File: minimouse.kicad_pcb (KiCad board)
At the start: 2 copper layers, 90 x 85 mm, 22 parts, among them J1 Conn_ARM_JTAG_SWD_10, J5 Conn_01x02, M1 N20_encoder, M2 N20_encoder, U1 STM32F030C8Tx, U4 HC-SR04

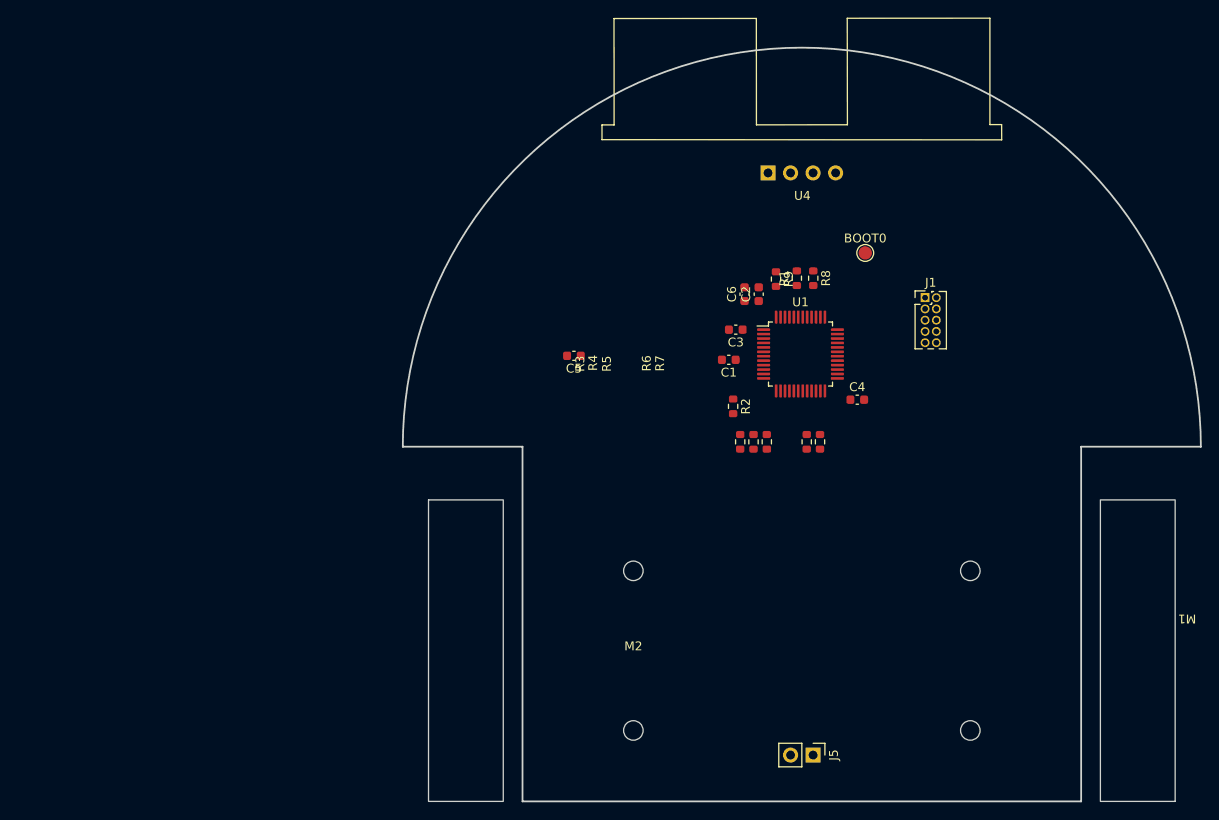
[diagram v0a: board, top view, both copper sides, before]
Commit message: TP2
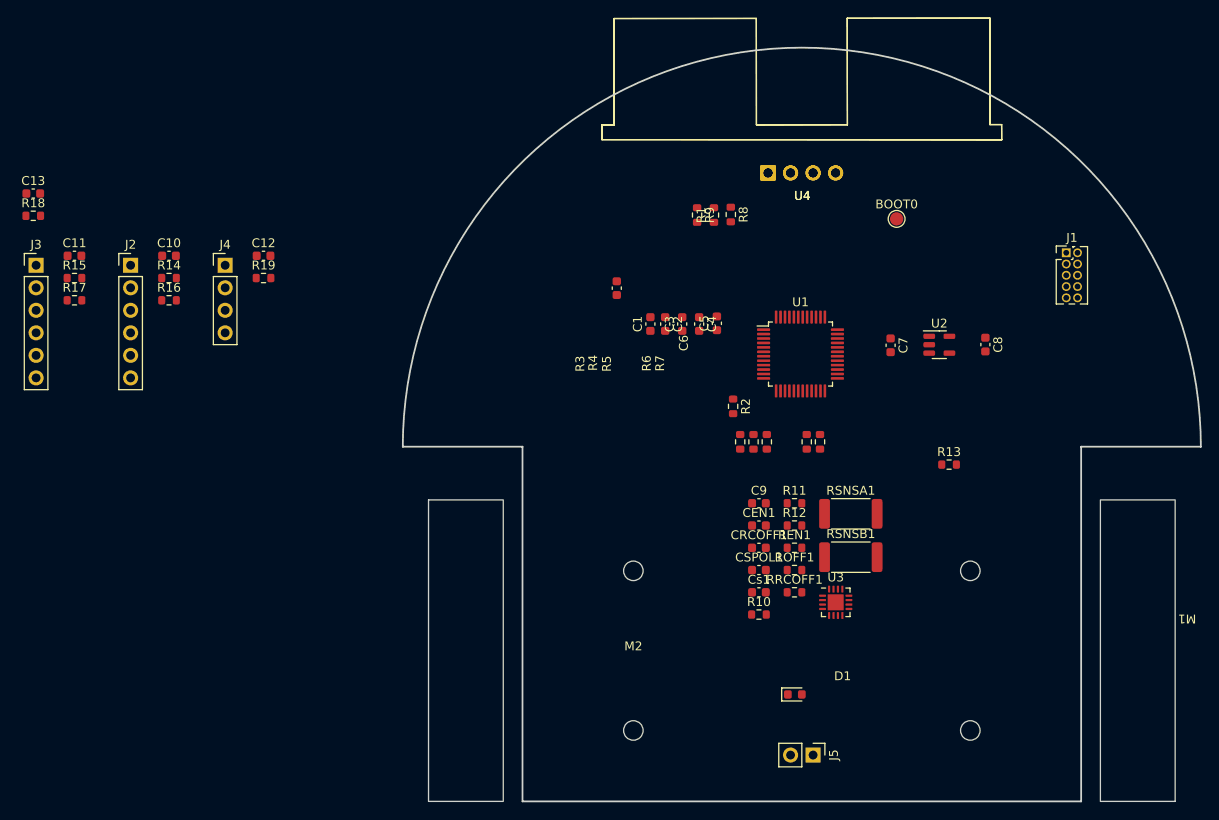
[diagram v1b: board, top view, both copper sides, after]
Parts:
- added C10: 2.2u, Capacitor_SMD:C_0603_1608Metric, F.Cu at (78.6, 78.5)
- added C11: 2.2u, Capacitor_SMD:C_0603_1608Metric, F.Cu at (68.0, 78.5)
- added C12: C, Capacitor_SMD:C_0603_1608Metric, F.Cu at (89.3, 78.5)
- added C13: 2.2u, Capacitor_SMD:C_0603_1608Metric, F.Cu at (63.3, 71.5)
- added C7: 1uF, Capacitor_SMD:C_0603_1608Metric, F.Cu at (160.0, 88.6)
- added C8: 1uF, Capacitor_SMD:C_0603_1608Metric, F.Cu at (170.7, 88.5)
- added C9: C, Capacitor_SMD:C_0603_1608Metric, F.Cu at (145.2, 106.4)
- added CEN1: 10nF, Capacitor_SMD:C_0603_1608Metric, F.Cu at (145.2, 108.9)
- added CRCOFF1: 22nF, Capacitor_SMD:C_0603_1608Metric, F.Cu at (145.2, 111.4)
- added CSPOL1: 22uF, Capacitor_SMD:C_0603_1608Metric, F.Cu at (145.2, 113.9)
- added Cs1: 2.2uF, Capacitor_SMD:C_0603_1608Metric, F.Cu at (145.2, 116.4)
- added D1: LED, LED_SMD:LED_0603_1608Metric, F.Cu at (149.2, 127.9)
- added J2: Conn_01x06, Connector_PinHeader_2.54mm:PinHeader_1x06_P2.54mm_Vertical, F.Cu at (74.3, 79.5)
- added J3: Conn_01x06, Connector_PinHeader_2.54mm:PinHeader_1x06_P2.54mm_Vertical, F.Cu at (63.6, 79.5)
- added J4: Conn_01x04, Connector_PinHeader_2.54mm:PinHeader_1x04_P2.54mm_Vertical, F.Cu at (85.0, 79.5)
- added R10: 10K, Resistor_SMD:R_0603_1608Metric, F.Cu at (145.2, 118.9)
- added R11: 10K, Resistor_SMD:R_0603_1608Metric, F.Cu at (149.2, 106.4)
- added R12: R, Resistor_SMD:R_0603_1608Metric, F.Cu at (149.2, 108.9)
- added R13: R, Resistor_SMD:R_0603_1608Metric, F.Cu at (166.6, 102.0)
- added R14: 100, Resistor_SMD:R_0603_1608Metric, F.Cu at (78.6, 81.0)
- added R15: 100, Resistor_SMD:R_0603_1608Metric, F.Cu at (68.0, 81.0)
- added R16: 100, Resistor_SMD:R_0603_1608Metric, F.Cu at (78.6, 83.5)
- added R17: 100, Resistor_SMD:R_0603_1608Metric, F.Cu at (68.0, 83.5)
- added R18: 100, Resistor_SMD:R_0603_1608Metric, F.Cu at (63.3, 74.0)
- added R19: 100, Resistor_SMD:R_0603_1608Metric, F.Cu at (89.3, 81.0)
- added REN1: 18K, Resistor_SMD:R_0603_1608Metric, F.Cu at (149.2, 111.4)
- added ROFF1: 47K, Resistor_SMD:R_0603_1608Metric, F.Cu at (149.2, 113.9)
- added RRCOFF1: 1K, Resistor_SMD:R_0603_1608Metric, F.Cu at (149.2, 116.4)
- added RSNSA1: 330 m, Resistor_SMD:R_2512_6332Metric, F.Cu at (155.5, 107.6)
- added RSNSB1: 330m, Resistor_SMD:R_2512_6332Metric, F.Cu at (155.5, 112.5)
- added U2: LP5907MFX-1.2, Package_TO_SOT_SMD:SOT-23-5, F.Cu at (165.5, 88.5)
- added U3: STSPIN240, Package_DFN_QFN:VQFN-16-1EP_3x3mm_P0.5mm_EP1.8x1.8mm, F.Cu at (153.8, 117.5)
- added U4: HC-SR04, minimouse:HC-SR04, F.Cu at (150.0, 69.1)
- moved C4 19.8 mm to (138.4, 86.2), turned to -90 degrees
- moved J1 16.7 mm to (179.8, 78.1)
- moved C5 16.5 mm to (140.4, 86.1), turned to 90 degrees
- moved C6 14.4 mm to (129.1, 82.1), turned to -90 degrees
- moved R1 11.8 mm to (140.1, 73.9)
- moved R8 11.8 mm to (142.0, 73.8)
- moved R9 11.5 mm to (138.2, 73.9)
- moved C2 11.1 mm to (134.6, 86.2), turned to -90 degrees
- moved C1 9.72 mm to (132.9, 86.2), turned to 90 degrees
- moved C3 6.07 mm to (136.5, 86.2), turned to 90 degrees
- moved BOOT0 5.22 mm to (160.7, 74.3)
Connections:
- R2 pad 2: /mcu/TIM15_CH1 -> /mcu/OUT_A4
- R6 pad 1: /mcu/OUT_B0 -> /motor_control/STBY_RESET
- R8 pad 1: /mcu/UART1_TX -> /external_uart/EXT_UART_RX
- U1 pad 43: /mcu/UART1_RX -> /external_uart/EXT_UART_TX
